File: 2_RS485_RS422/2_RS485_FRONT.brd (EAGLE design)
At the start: 71.5 x 24 mm, 3 parts

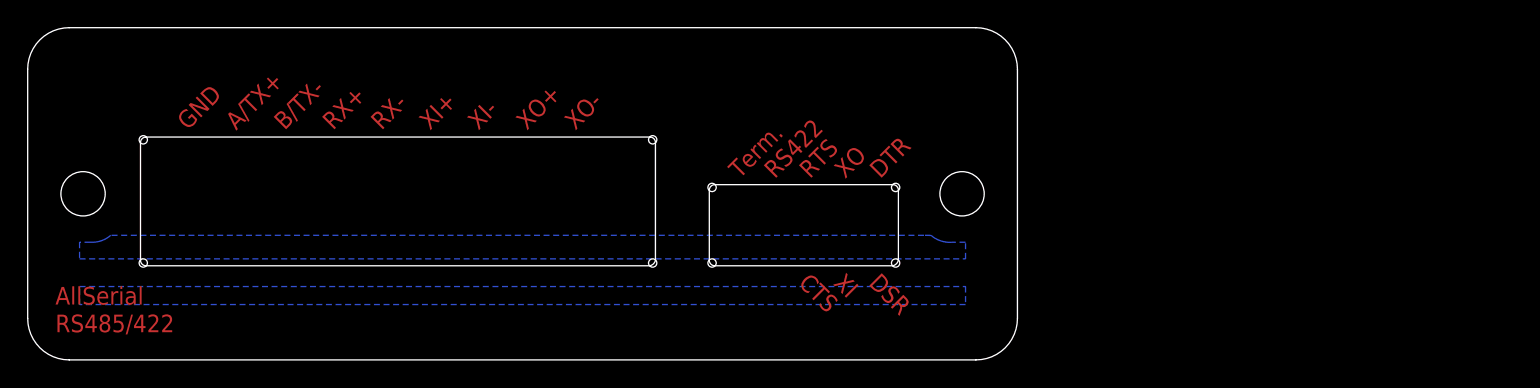
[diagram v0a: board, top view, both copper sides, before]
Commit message: Cleanup, front with lib elements
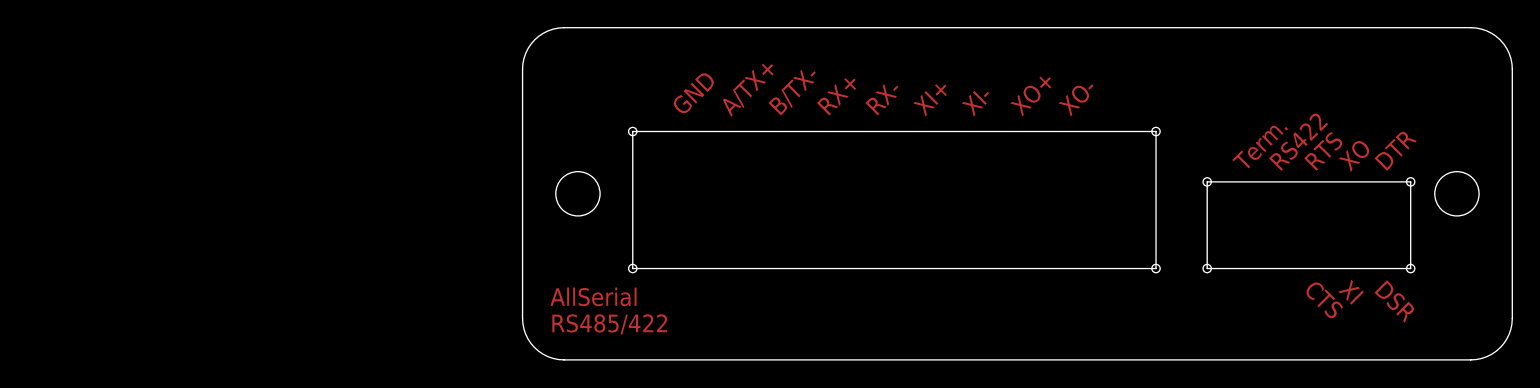
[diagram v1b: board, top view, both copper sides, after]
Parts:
- removed E$1: (no value), AllSerialv2:PANEL
- removed E$2: (no value), AllSerialv2:RIA_AKL182-10
- removed E$3: (no value), AllSerialv2:LSTB-05-2
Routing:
- removed copper zone on layer 16, net S$1
- removed copper zone on layer 16, net S$2
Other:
- outline, holes or cut-outs redrawn
- board text added: "AllSerial RS485/422"
- board text removed: "AllSerial RS485/422 v1.1 46/18"
- board text removed: "RS485/422"
